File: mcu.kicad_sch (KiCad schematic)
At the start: 6 parts, among them Q4 NMOS, U4 ESP32-S3-WROOM-1

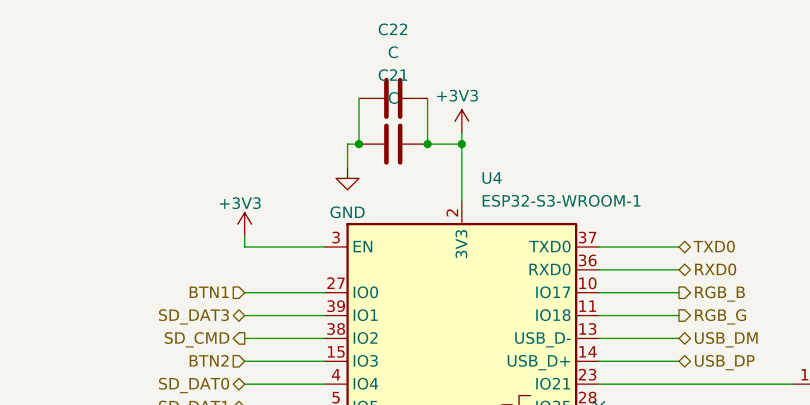
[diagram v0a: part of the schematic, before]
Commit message: update pcb and schematic
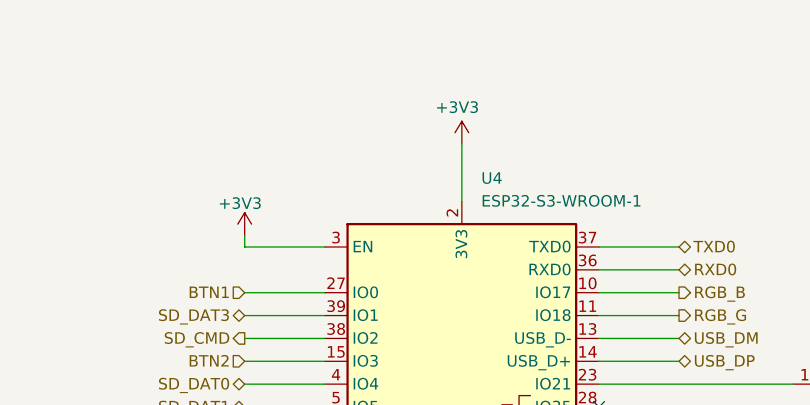
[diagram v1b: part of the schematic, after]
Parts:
- removed C21, C22: C, Capacitor_SMD:C_0805_2012Metric, symbol Device:C
